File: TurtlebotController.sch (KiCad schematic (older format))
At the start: 14 parts, among them J1 Raspberry_Pi_2_3, U1 Teensy4.0, U2 MinIMU-9_V5, U7 UltimateSensorFusion_MPU9250_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

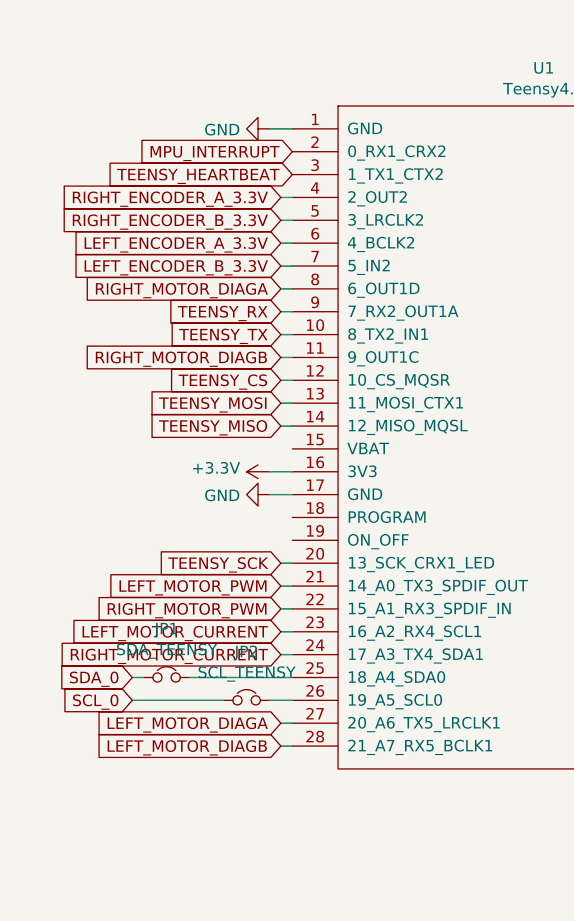
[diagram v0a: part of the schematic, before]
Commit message: Some fixes
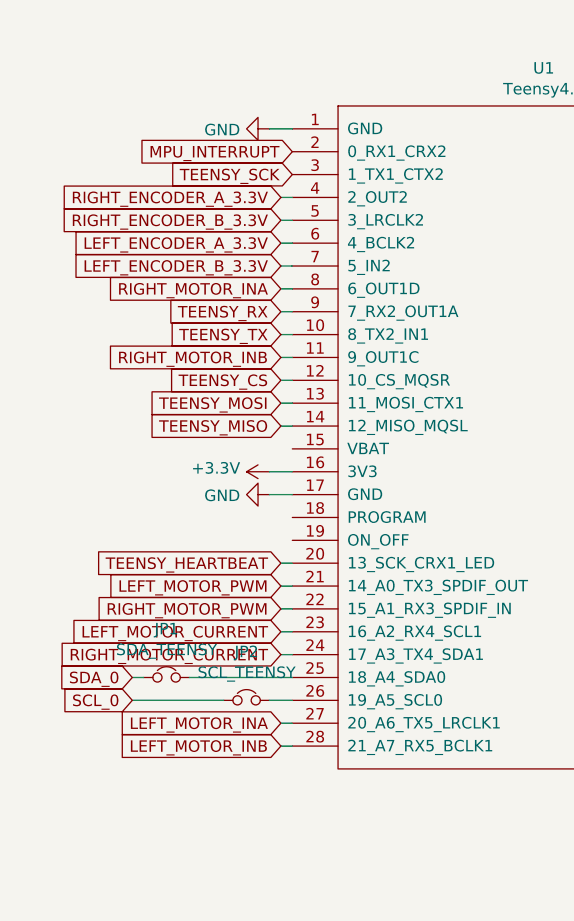
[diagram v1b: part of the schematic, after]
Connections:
- net TEENSY_HEARTBEAT: now also U1.20 (13_SCK_CRX1_LED); no longer U1.3 (1_TX1_CTX2)
- net TEENSY_SCK: now also U1.3 (1_TX1_CTX2); no longer U1.20 (13_SCK_CRX1_LED)
- net LEFT_MOTOR_DIAGA renamed LEFT_MOTOR_INA
- net LEFT_MOTOR_DIAGB renamed LEFT_MOTOR_INB
- net RIGHT_MOTOR_DIAGA renamed RIGHT_MOTOR_INA
- net RIGHT_MOTOR_DIAGB renamed RIGHT_MOTOR_INB
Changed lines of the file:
@@
 	1600 3450 1650 3450
 Text GLabel 1600 3750 0    50   Input ~ 0
-LEFT_MOTOR_DIAGA
+LEFT_MOTOR_INA
 Text GLabel 1600 3850 0    50   Input ~ 0
-LEFT_MOTOR_DIAGB
+LEFT_MOTOR_INB
 Text GLabel 1600 1850 0    50   Input ~ 0
-RIGHT_MOTOR_DIAGA
+RIGHT_MOTOR_INA
 Text GLabel 1600 2150 0    50   Input ~ 0
-RIGHT_MOTOR_DIAGB
+RIGHT_MOTOR_INB
 Wire Wire Line
 	1600 1650 1650 1650
@@
 Wire Wire Line
 	1600 2250 1650 2250
-Text GLabel 1600 3050 0    50   Input ~ 0
+Text GLabel 1650 1350 0    50   Input ~ 0
 TEENSY_SCK
 Wire Wire Line
@@
 Wire Wire Line
 	7000 3750 6900 3750
-Text GLabel 1650 1350 0    50   Input ~ 0
+Text GLabel 1600 3050 0    50   Input ~ 0
 TEENSY_HEARTBEAT
 Wire Wire Line
